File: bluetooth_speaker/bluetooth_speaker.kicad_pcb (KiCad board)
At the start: 2 copper layers, 70 x 44 mm, 47 parts, among them J1 Conn_Coaxial, J2 USB_C_Receptacle_USB2.0_16P, J3 282836-4, J5 Conn_01x04_Pin, Q1 SS8050-G, Q2 SS8050-G, U1 MAX98357A, U2 XL4015, U3 CP2102N-A01-GQFN28, U4 ESP32-D0WD-V3, Y1 40MHz(±10 ppm)

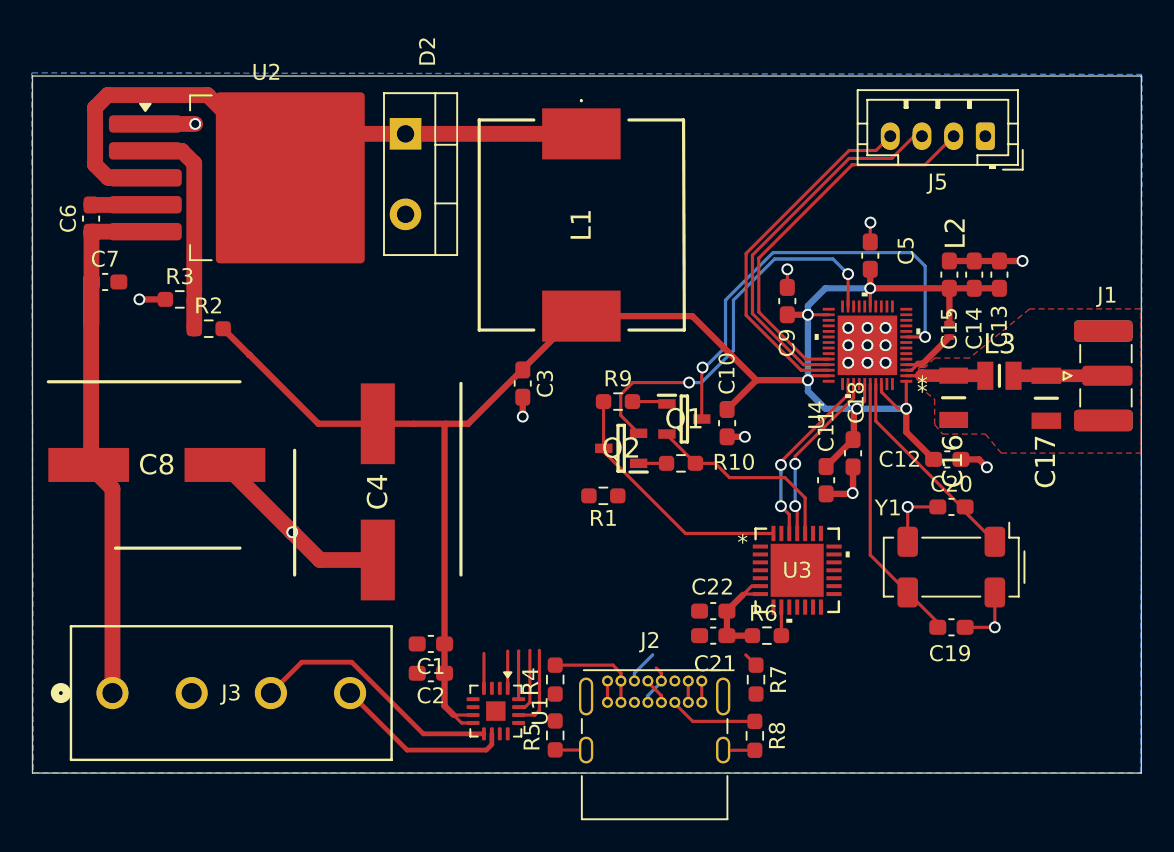
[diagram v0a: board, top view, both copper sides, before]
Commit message: Completed the PCB design
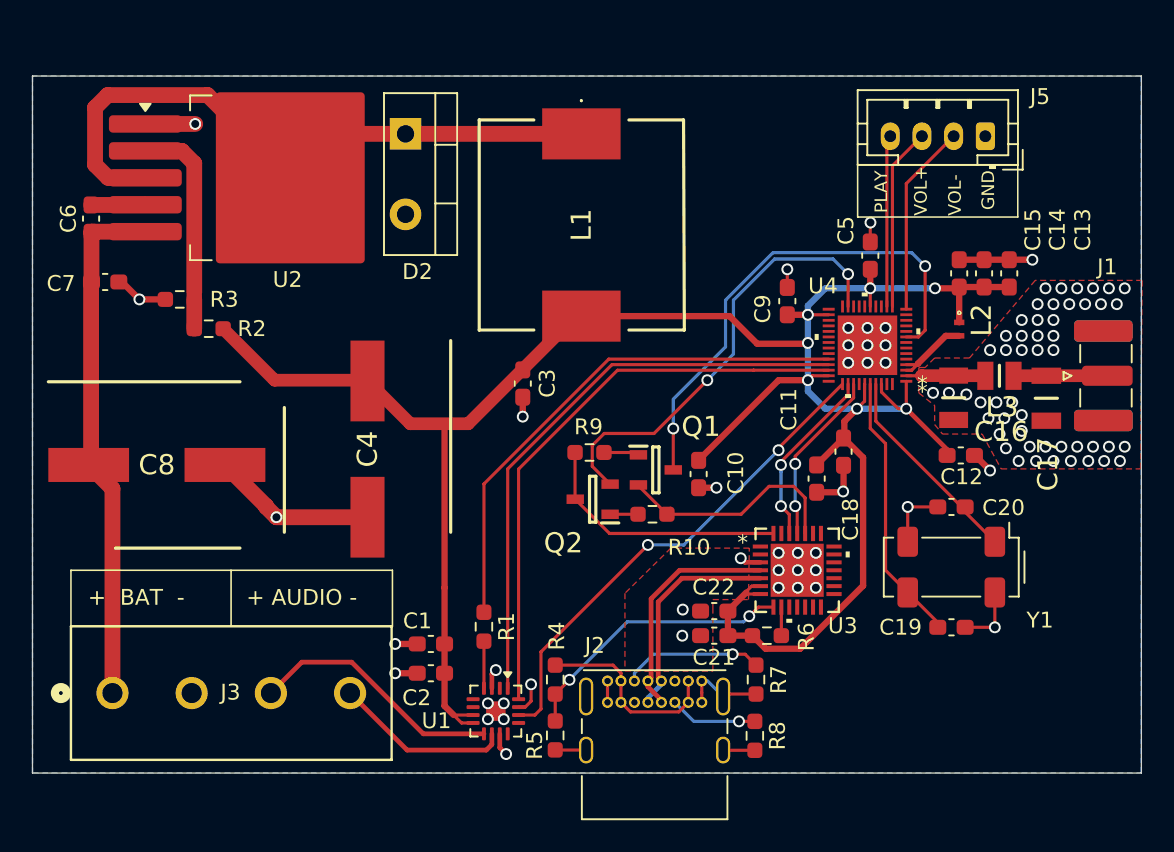
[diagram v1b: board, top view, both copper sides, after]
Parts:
- moved R1 11.2 mm to (142.1, 116.4), turned to -90 degrees
- moved R10 3.68 mm to (152.7, 109.3)
- moved Q2 3.68 mm to (148.9, 108.3)
- moved C10 3.68 mm to (155.6, 106.7)
- moved Q1 3.68 mm to (152.9, 106.5)
- moved R9 3.68 mm to (148.7, 105.4)
- moved C4 2.78 mm to (134.7, 105.2)
- moved C12 0.89 mm to (172.2, 105.5)
- moved C13 0.63 mm to (175.2, 94.1)
- moved C14 0.63 mm to (173.6, 94.1)
- moved C15 0.63 mm to (172.1, 94.1)
- moved L2 0.63 mm to (172.1, 97.6)
- moved C11 0.61 mm to (163.1, 107.0)
- moved C18 0.61 mm to (164.8, 105.3)
- moved C21 0.06 mm to (156.6, 116.9)
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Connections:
- U4 pad 14: /LRCLK -> /BTN_VOL_DOWN
- U4 pad 15: /BCLK -> /BTN_VOL_UP
- U4 pad 16: /SD_MODE -> /BTN_PLAY
- U4 pad 34: /BTN_VOL_DOWN -> /SD_MODE
- U4 pad 35: /BTN_VOL_UP -> /DATA
- U4 pad 36: /BTN_PLAY -> /BCLK
- U4 pad 39: /DATA -> /LRCLK
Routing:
- net /DATA: track 2.35 -> 36.8 mm
- net /BCLK: track 3.04 -> 36.7 mm
- net /SD_MODE: track 0.00 -> 33.1 mm
- net /LRCLK: track 5.23 -> 31.3 mm, vias 0 -> 2
- net +3.3V: track 124.4 -> 149.8 mm, vias 5 -> 7
- net Net-(U3-VBUS): track 0.00 -> 17.8 mm, vias 0 -> 2
- net /USB-UART Converter/USB_D+: track 1.74 -> 14.7 mm
- net /BTN_VOL_DOWN: track 24.5 -> 12.2 mm
- net /BTN_VOL_UP: track 23.7 -> 11.5 mm
- net /BTN_PLAY: track 22.7 -> 10.8 mm
- net /USB-UART Converter/USB_D-: track 2.66 -> 13.9 mm
- net GND: track 50.4 -> 58.6 mm, vias 21 -> 92
- net Net-(J2-CC1): track 3.05 -> 8.95 mm, vias 0 -> 1
- net /USB-UART Converter/VBUS: track 7.55 -> 12.3 mm
- net /EN: track 28.1 -> 31.7 mm
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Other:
- board text added: "*"
- board text added: "+ AUDIO -"
- board text added: "+ BAT -"
- board text added: "GND"
- board text added: "PLAY"
- board text added: "VOL+"
- board text added: "VOL-"
